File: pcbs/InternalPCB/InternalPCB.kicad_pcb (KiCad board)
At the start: 2 copper layers, 16 parts, among them J1 Conn_01x20, J10 694106301002, J2 Conn_01x20, J3 Conn_01x04_Pin, J4 Conn_01x04_Pin, J5 Conn_01x02_Pin, J6 Conn_01x04_Pin, J7 Conn_01x03_Pin, J8 Conn_01x05_Pin, J9 Conn_01x05_Pin, SW1 SW_Push, U1 Pico W, U2 Pico, U3 004-0-0013

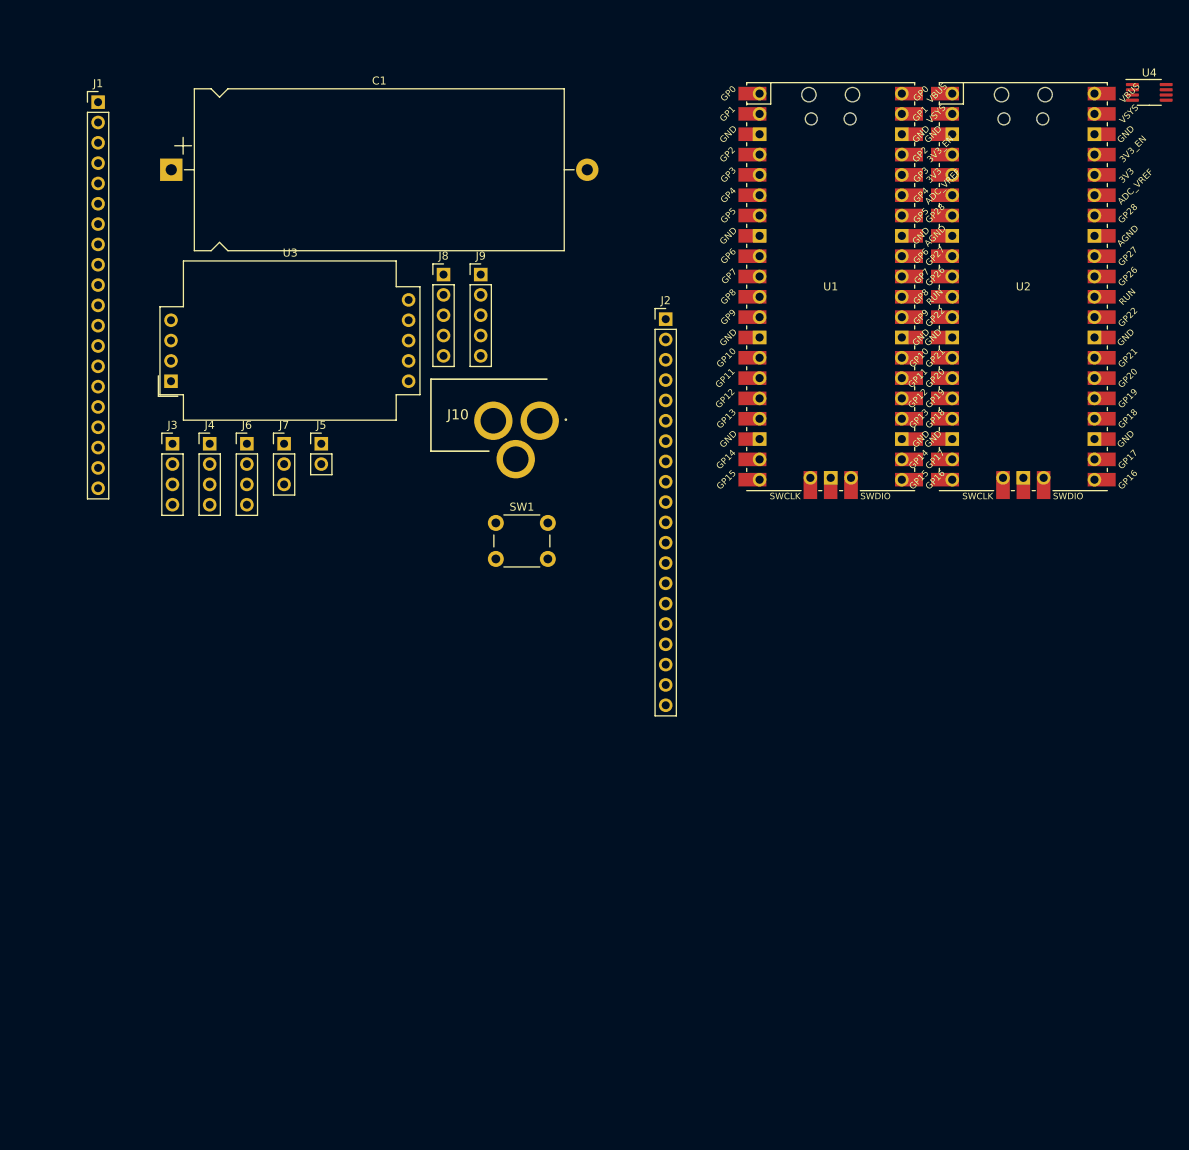
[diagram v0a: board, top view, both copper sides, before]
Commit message: Innenmodul erstes funktionales PCB
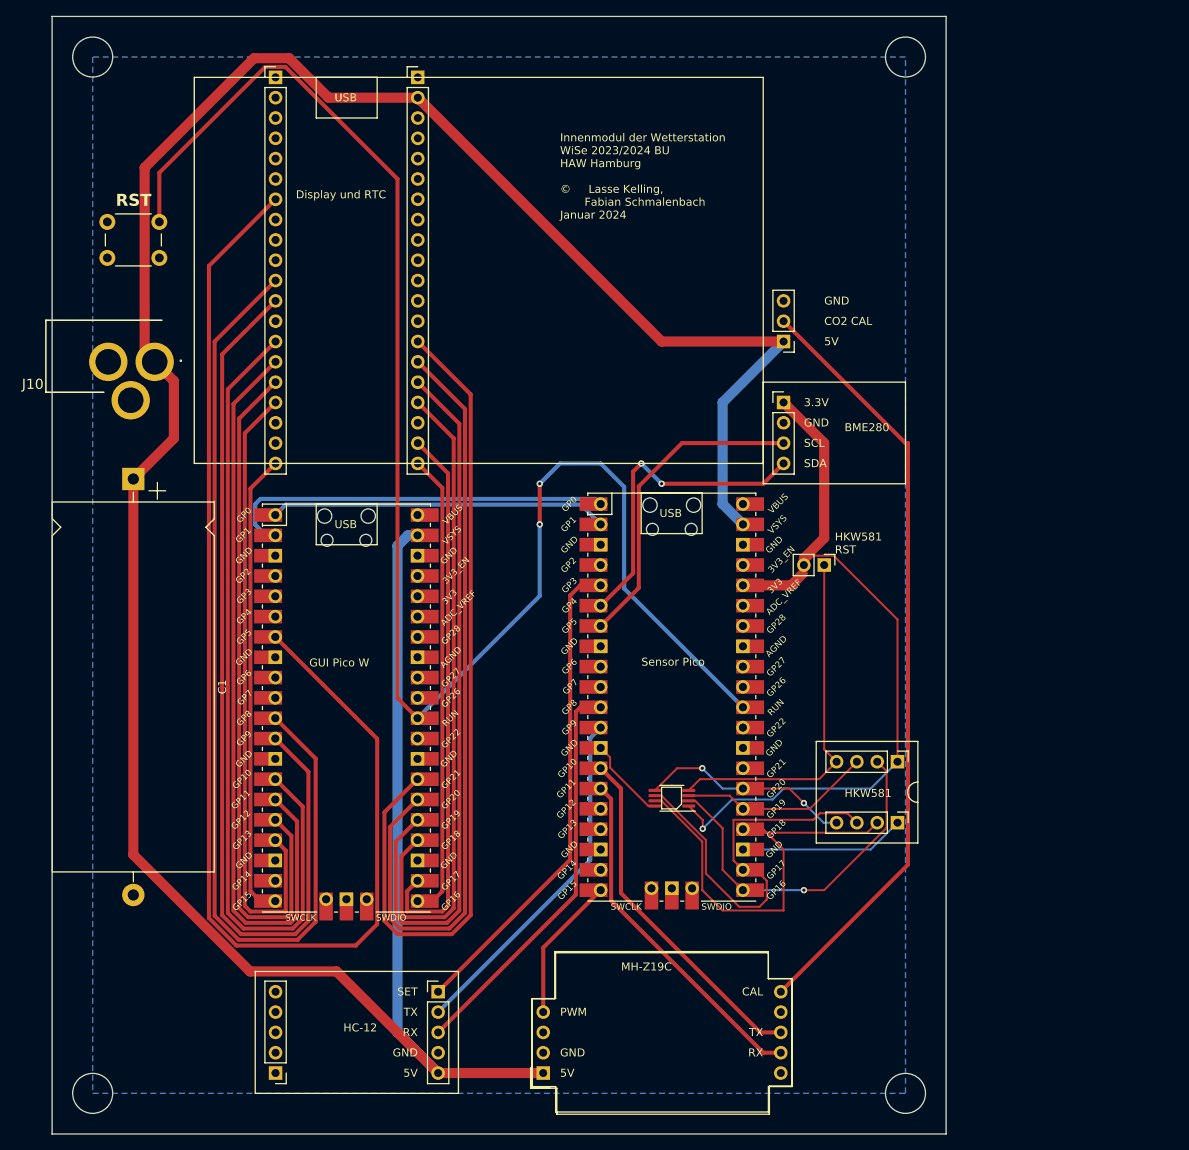
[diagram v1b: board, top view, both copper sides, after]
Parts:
- moved U4 106.5 mm to (102.9, 130.7), turned to 180 degrees
- moved J9 103.1 mm to (53.3, 165.1), turned to 180 degrees
- moved J3 99.0 mm to (131.1, 126.2), turned to -90 degrees
- moved U3 98.2 mm to (86.8, 165.1)
- moved J4 98.2 mm to (131.1, 133.8), turned to -90 degrees
- moved J8 89.7 mm to (73.7, 154.9)
- moved U1 80.2 mm to (62.2, 119.5)
- moved U2 67.6 mm to (102.9, 118.1)
- moved J6 67.3 mm to (116.8, 81.3)
- moved J5 64.7 mm to (121.9, 101.6), turned to -90 degrees
- moved J7 63.7 mm to (116.8, 73.7), turned to 180 degrees
- moved SW1 61.4 mm to (32.3, 58.7)
- moved J2 57.4 mm to (53.3, 40.6)
- moved J10 48.7 mm to (24.6, 80.0)
- moved J1 40.1 mm to (71.1, 40.6)
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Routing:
- net +5V: track 0.00 -> 350.4 mm
- net PICO_RESET: track 0.00 -> 197.8 mm, vias 0 -> 2
- net SDIO_CLK: track 0.00 -> 158.0 mm
- net LCD_DC: track 0.00 -> 124.9 mm
- net LCD_CS: track 0.00 -> 116.5 mm
- net D2: track 0.00 -> 106.3 mm
- net CLK: track 0.00 -> 103.4 mm
- net D1: track 0.00 -> 98.3 mm
- net Net-(J7-Pin_2): track 0.00 -> 97.0 mm
- net 3.3V: track 0.00 -> 96.2 mm, vias 0 -> 1
- net MOSI: track 0.00 -> 95.4 mm
- net D0: track 0.00 -> 90.3 mm
- net MISO: track 0.00 -> 87.4 mm
- net SDIO_CMD: track 0.00 -> 82.3 mm
- net LCD_BL: track 0.00 -> 79.4 mm
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- added copper zone on B.Cu, net GND
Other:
- board outline added: 111.8 x 139.7 mm
- board text added: "3.3V"
- board text added: "5V"
- board text added: "BME280"
- board text added: "CAL"
- board text added: "CO2 CAL"
- board text added: "Display und RTC"
- board text added: "GND"
- board text added: "GUI Pico W"
- board text added: "HC-12"
- board text added: "HKW581"
- board text added: "HKW581 RST"
- board text added: "Innenmodul der Wetterstation WiSe 2023/2024 BU HAW Hamburg © Lasse Kelling, Fabian Schmalenbach Januar 2024"
- board text added: "MH-Z19C"
- board text added: "PWM"
- board text added: "RST"
- board text added: "RX"
- board text added: "SCL"
- board text added: "SDA"
- board text added: "SET"
- board text added: "Sensor Pico"
- board text added: "TX"
- board text added: "USB"
